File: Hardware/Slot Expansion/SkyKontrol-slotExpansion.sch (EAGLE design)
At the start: 23 parts, among them J4 SBH11-PBPC-D05, T1 MMBT3904, T2 MMBT3904, U1 PIC12F1822-E/SN

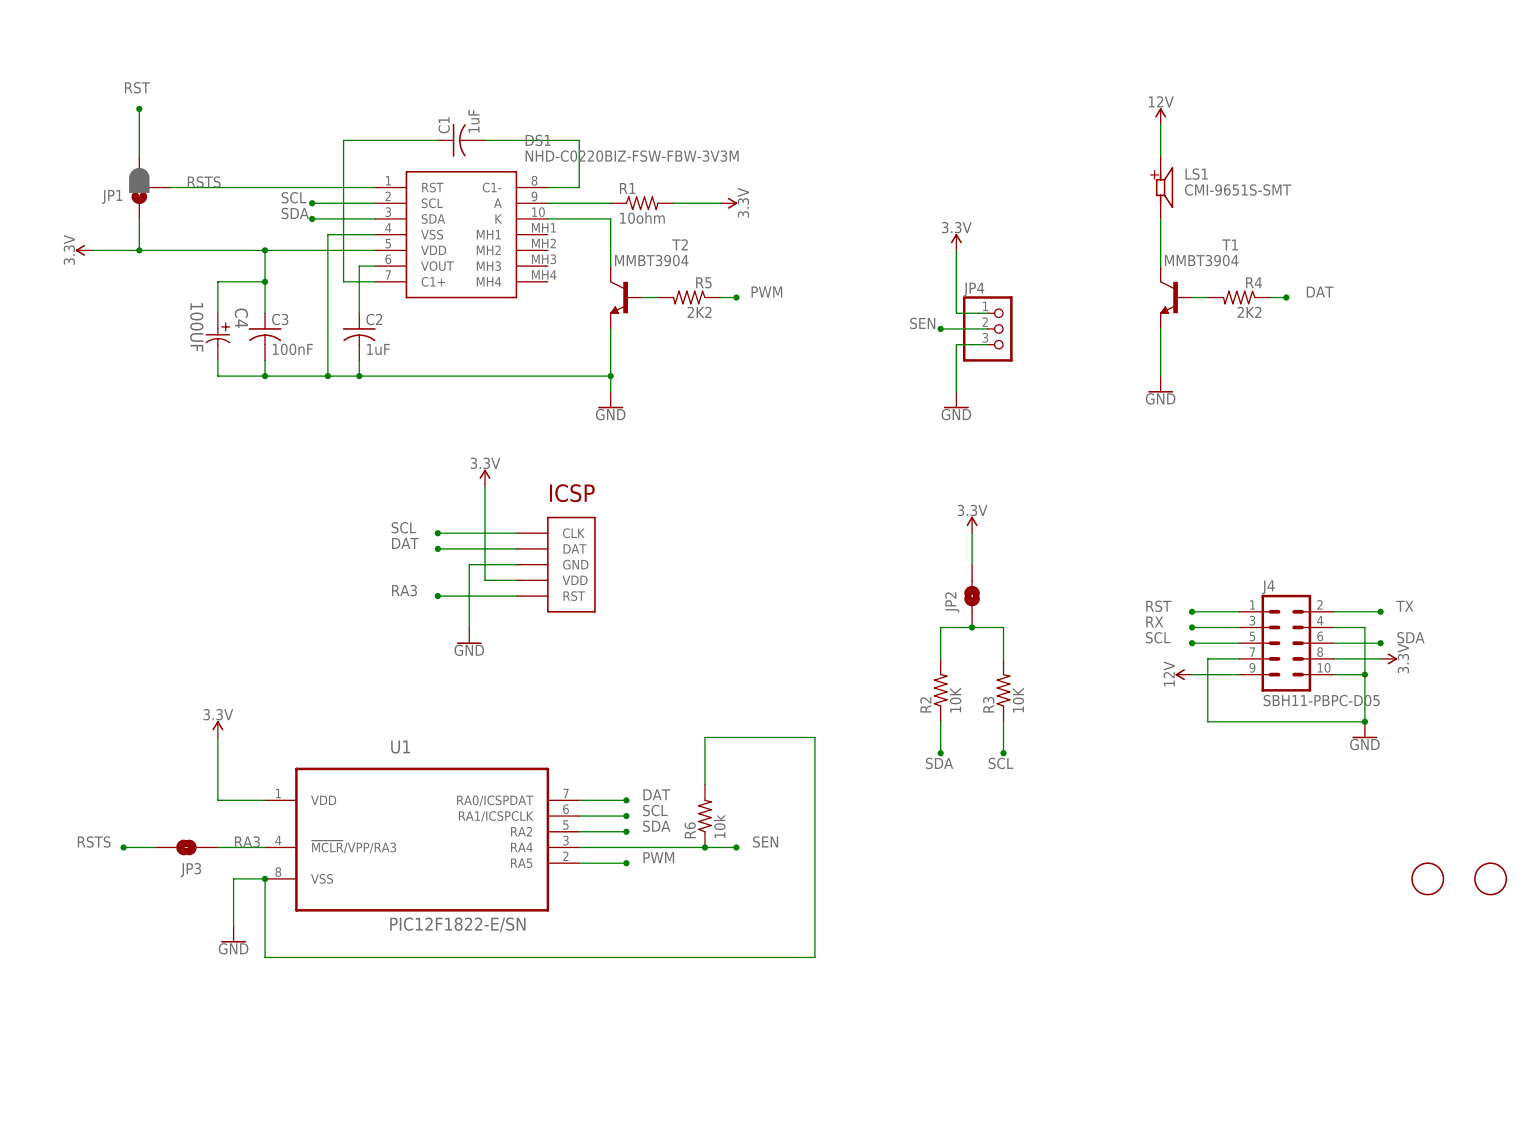
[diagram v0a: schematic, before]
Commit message: documentation add
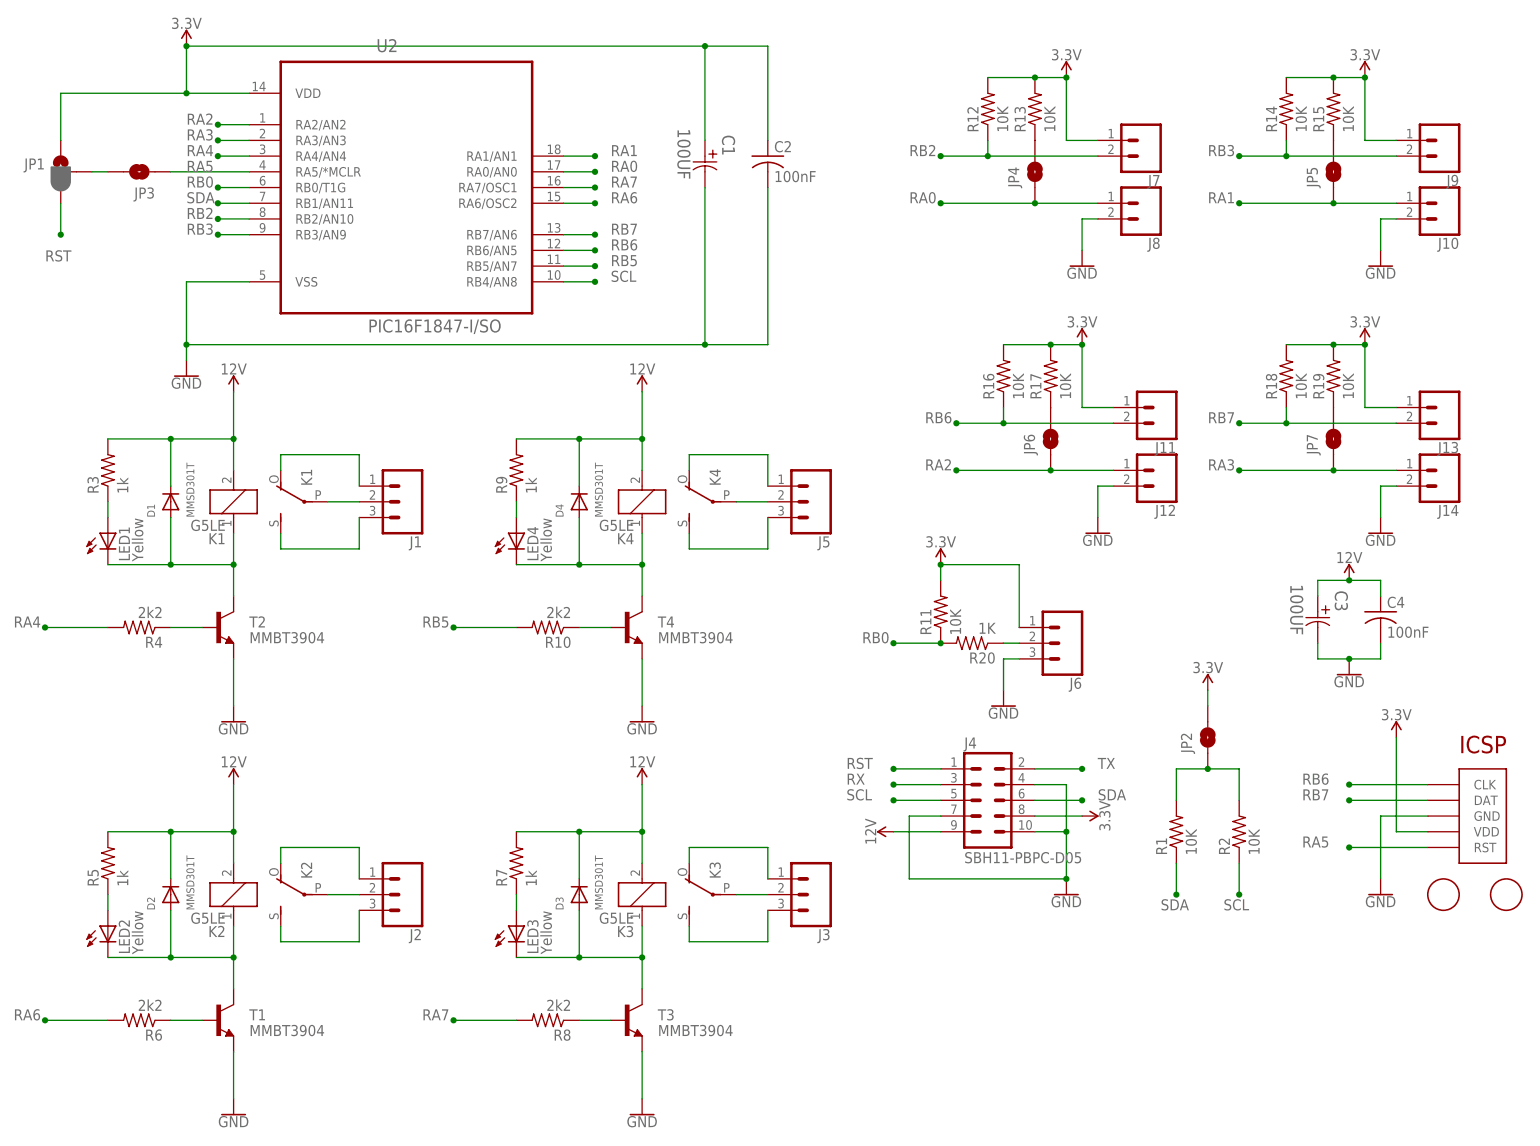
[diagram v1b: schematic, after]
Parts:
- removed DS1: NHD-C0220BIZ-FSW-FBW-3V3M, NHD-C0220BIZ-FSW-FBW-3V3M:NHD-C0220BIZ-FSW-FBW-3V3M
- removed LS1: CMI-9651S-SMT, CMI-9651S-SMT:CMI-9651S-SMT
- removed U1: PIC12F1822-E/SN, Microchip-PIC12F1822-E_SN:PIC12F1822-E/SN
- added D1, D2, D3, D4: MMSD301T, adafruit:DIODESOD-123
- added J1, J2, J3, J5, J6: (no value), SparkFun-Connectors:CONN_03-SCREW-5MM
- added J10, J11, J12, J13, J14, J7, J8, J9: (no value), SparkFun-Connectors:CONN_025MM
- added JP5, JP6, JP7: JUMPER-SMT_2_NO_SILK, SparkFun-Jumpers:JUMPER-SMT_2_NO_SILK
- added K1, K2, K3, K4: G5LE, relay:G5LE
- added LED1, LED2, LED3, LED4: Yellow, adafruit:LEDCHIPLED_1206
- added R10, R8: 2k2, adafruit:R-US_R0805
- added R11, R12, R13, R14, R15, R16, R17, R18, R19: 10K, adafruit:R-US_R0805
- added R20: 1K, adafruit:R-US_R0805
- added R7, R9: 1k, adafruit:R-US_R0805
- added T3, T4: MMBT3904, transistor:MMBT3904LT1-NPN-SOT23-BEC
- added U2: PIC16F1847-I/SO, PIC 16F1847:PIC16F1847-I/SO
- C1: value 1uF -> 100UF; device adafruit:C-USC0603K -> Panasonic-EEEFT_EEEH:EEE-HA1E101XP-CASE-D8
- C2: value 1uF -> 100nF
- C3: value 100nF -> 100UF; device adafruit:C-USC0603K -> Panasonic-EEEFT_EEEH:EEE-HA1E101XP-CASE-D8
- C4: value 100UF -> 100nF; device Panasonic-EEEFT_EEEH:EEE-HA1E101XP-CASE-D8 -> adafruit:C-USC0603K
- JP4: value (none) -> JUMPER-SMT_2_NO_SILK; device adafruit:PINHD-1X3CB -> SparkFun-Jumpers:JUMPER-SMT_2_NO_SILK
- R1: value 10ohm -> 10K
- R3: value 10K -> 1k
- R4: value 2K2 -> 2k2
- R5: value 2K2 -> 1k
- R6: value 10k -> 2k2
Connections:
- removed net DAT: R4.1, U$2.DAT, U1.RA0/ICSPDAT
- removed net PWM: R5.1, U1.RA5
- removed net RSTS: DS1.RST, JP1.2, JP3.2
- removed net SEN: JP4.2, R6.1, U1.RA4
- new net N$13: LED1.A, R3.1
- new net N$14: R4.1, T2.B
- new net N$15: J6.2, R20.1
- new net N$16: J2.1, K22.O
- new net N$18: LED2.A, R5.1
- new net N$21: J3.2, K32.P
- new net N$22: J3.3, K32.S
- new net N$23: J3.1, K32.O
- new net N$24: D3.A, K31.1, LED3.C, T3.C
- new net N$25: LED3.A, R7.1
- new net N$26: R8.1, T3.B
- new net N$28: J5.2, K42.P
- new net N$29: J5.3, K42.S
- new net N$30: J5.1, K42.O
- new net N$31: D4.A, K41.1, LED4.C, T4.C
- new net N$32: LED4.A, R9.1
- new net N$33: R10.1, T4.B
- new net N$37: JP4.2, R13.1
- new net N$39: JP5.2, R15.1
- new net N$40: JP6.2, R17.1
- new net N$41: JP7.2, R19.1
- new net N$9: D1.A, K11.1, LED1.C, T2.C
- new net RA0: J8.1, JP4.1, U2.RA0/AN0
- new net RA1: J10.1, JP5.1, U2.RA1/AN1
- new net RA2: J12.1, JP6.1, U2.RA2/AN2
- new net RA4: R4.2, U2.RA4/AN4
- new net RA5: JP3.1, U$2.RST, U2.RA5/*MCLR
- new net RA6: R6.2, U2.RA6/OSC2
- new net RA7: R8.2, U2.RA7/OSC1
- new net RB0: R11.1, R20.2, U2.RB0/T1G
- new net RB2: J7.2, R12.1, U2.RB2/AN10
- new net RB3: J9.2, R14.1, U2.RB3/AN9
- new net RB5: R10.2, U2.RB5/AN7
- new net RB6: J11.2, R16.1, U$2.CLK, U2.RB6/AN5
- new net RB7: J13.2, R18.1, U$2.DAT, U2.RB7/AN6
- net 12V: now also C3.1, C4.1, D1.C, D2.C, D3.C, D4.C, K11.2, K21.2, K31.2, K41.2, R3.2, R5.2, R7.2, R9.2; no longer LS1.P
- net 3.3V: now also C1.1, C2.1, J11.1, J13.1, J6.1, J7.1, J9.1, R11.2, R12.2, R13.2, R14.2, R15.2, R16.2, R17.2, R18.2, R19.2, U2.VDD; no longer C3.1, C4.1, DS1.VDD, JP4.1, R1.2, U1.VDD
- net GND: now also C1.2, J10.2, J12.2, J14.2, J6.3, J8.2, T3.E, T4.E, U2.VSS; no longer DS1.VSS, JP4.3, R6.2, U1.VSS
- net N$1: now also JP1.2, JP3.2; no longer C2.1, DS1.VOUT
- net N$10: now also J2.2, K22.P; no longer LS1.N, T1.C
- net N$12: now also J2.3, K22.S; no longer R4.2, T1.B
- net N$17: now also D2.A, K21.1, LED2.C, T1.C; no longer DS1.K, T2.C
- net N$19: now also R6.1, T1.B; no longer R5.2, T2.B
- net N$2: now also J1.2, K12.P; no longer C1.2, DS1.C1-
- net N$3: now also J1.3, K12.S; no longer C1.1, DS1.C1+
- net N$4: now also J1.1, K12.O; no longer DS1.A, R1.1
- net N$8: now also R1.2; no longer R3.2
- net RA3: now also J14.1, JP7.1, U2.RA3/AN3; no longer JP3.1, U$2.RST, U1.!MCLR!/VPP/RA3
- net SCL: now also R2.1, U2.RB4/AN8; no longer DS1.SCL, R3.1, U$2.CLK, U1.RA1/ICSPCLK
- net SDA: now also R1.1, U2.RB1/AN11; no longer DS1.SDA, R2.1, U1.RA2
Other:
- moved on the sheet: C2, J4, JP1, JP2, JP3, R1, R2, R3, R4, R5, R6, T1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
